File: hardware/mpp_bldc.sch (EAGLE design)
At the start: 86 parts, among them IC1 XMEGA16A4U, J2 USB-AB-MICROB-2, U1 LM3480IM3-5, U3 MIC5225-3.3, X1 PASSER-07, X2 PASSER-07

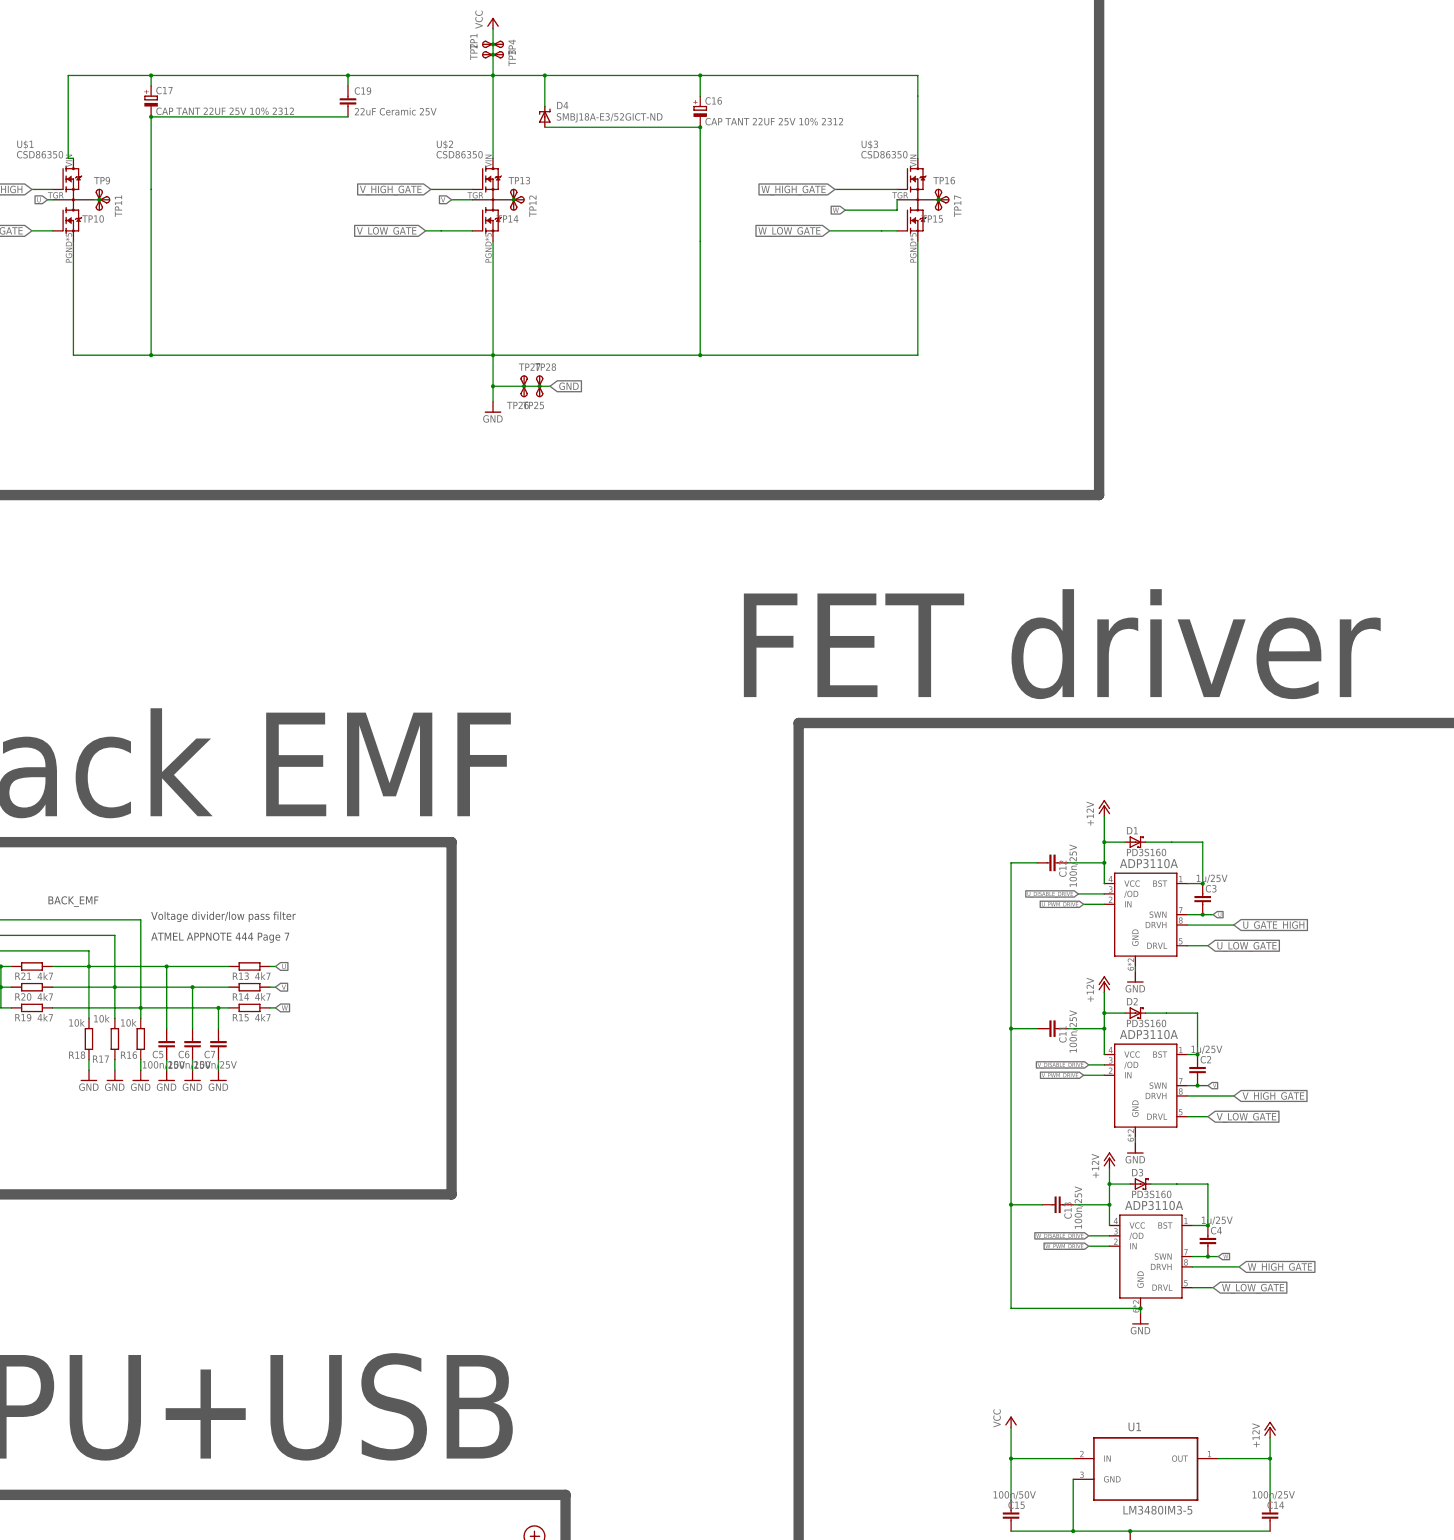
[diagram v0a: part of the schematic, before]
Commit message: tidy up
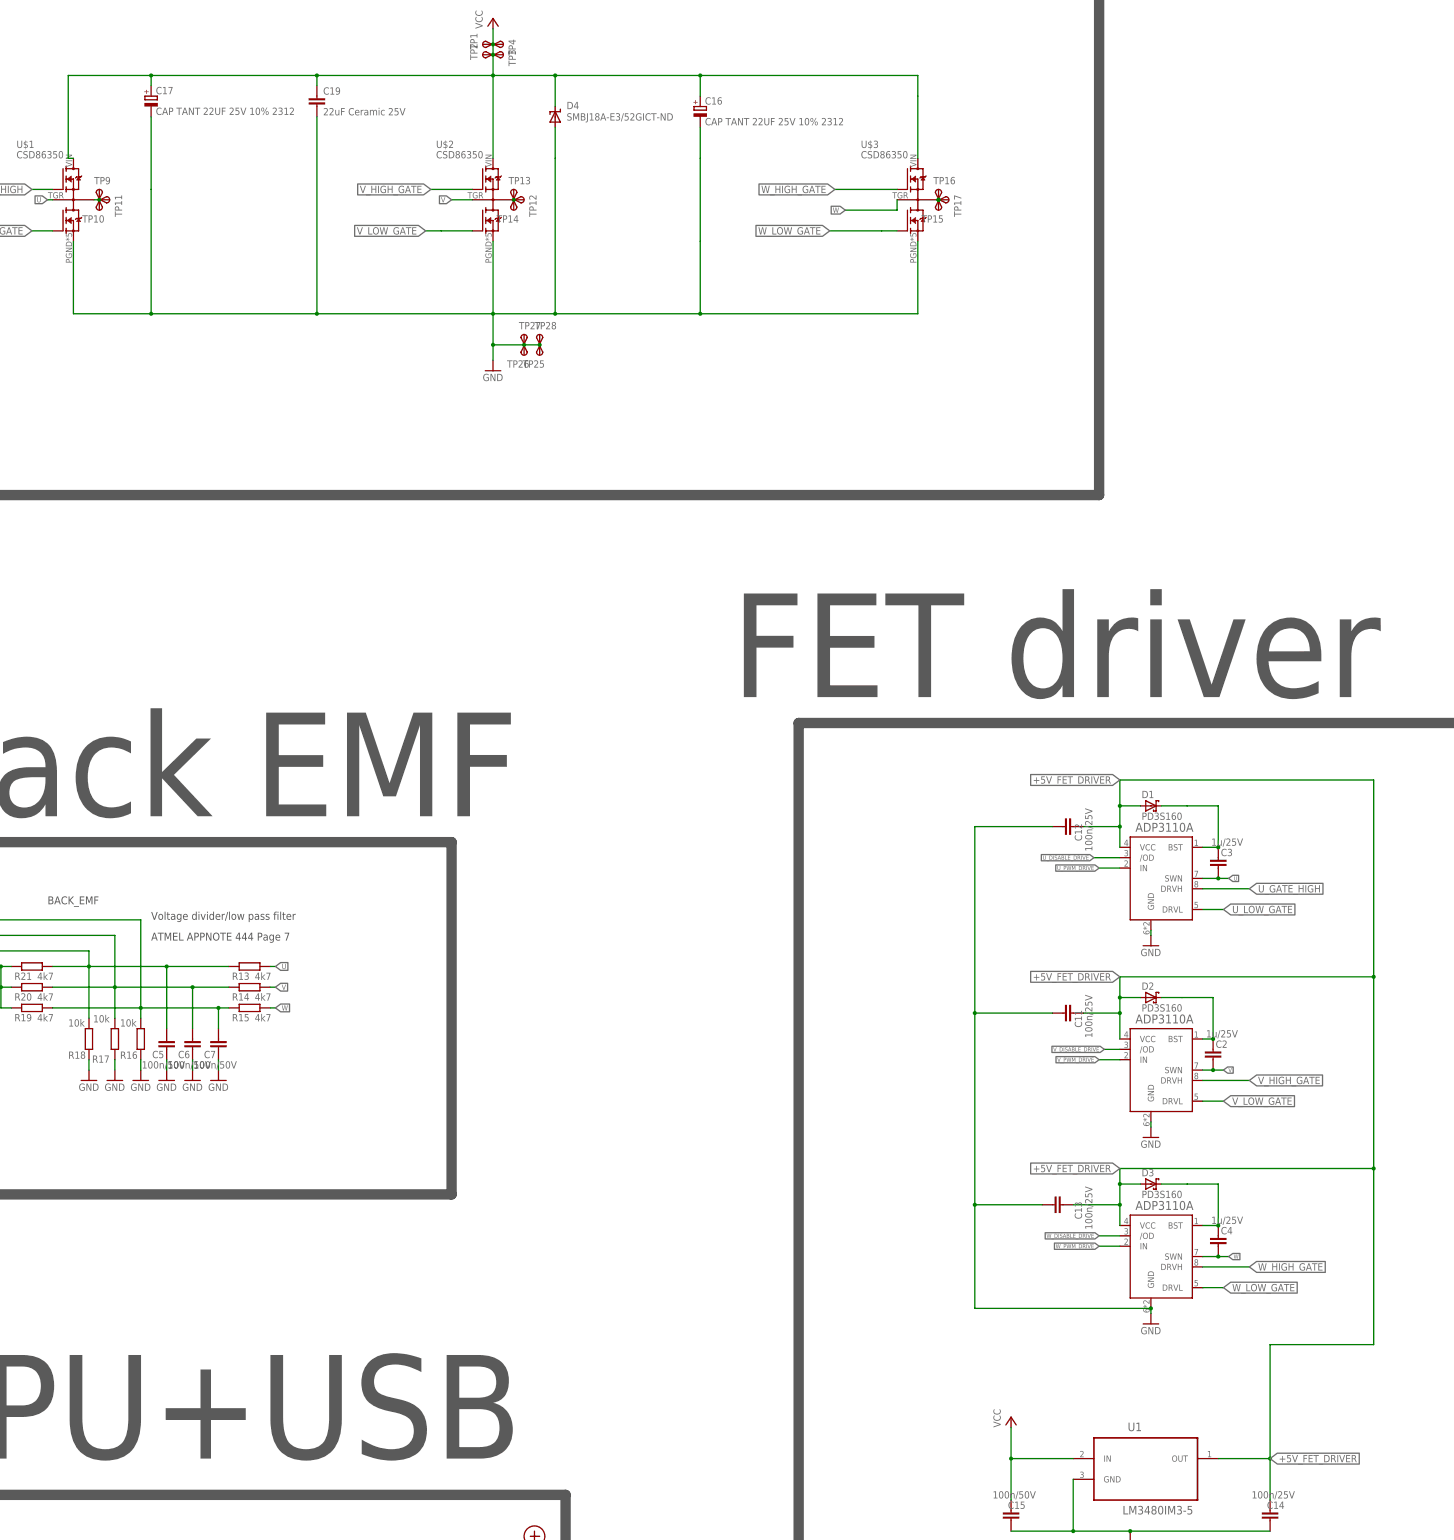
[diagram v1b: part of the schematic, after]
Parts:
- C5, C6, C7: value 100n/25V -> 100n/50V
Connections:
- net +12V renamed +5V_FET_DRIVER
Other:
- moved on the sheet: C11, C12, C19, C2, C3, C4, D1, D2, D3, D4, TP25, TP26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
